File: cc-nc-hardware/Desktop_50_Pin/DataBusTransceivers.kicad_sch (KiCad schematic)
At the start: 38 parts, among them J1 Conn_01x03_Male, Q1 AO3401A, Q2 AO3401A, U3 AMS1117-2.85, U4 LVT245, U5 LVT245, U6 LVT245, U9 LVT245

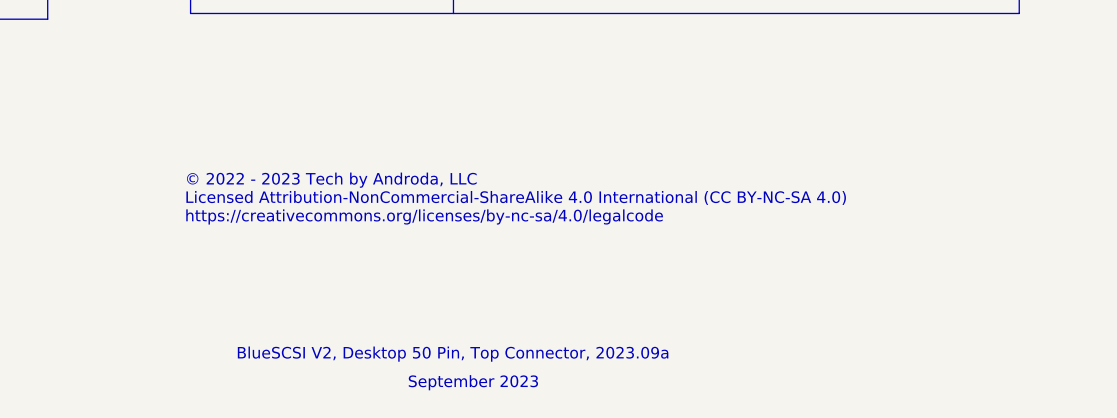
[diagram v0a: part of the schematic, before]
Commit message: Desktop 2023.10a design
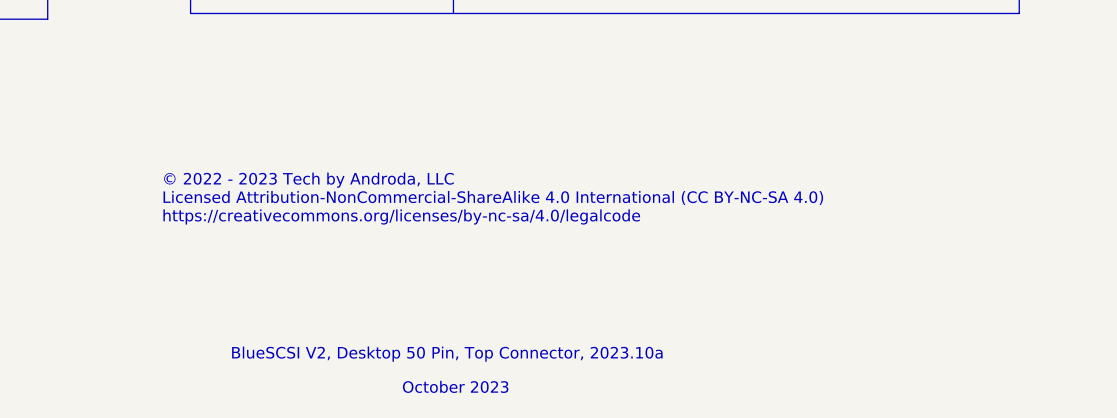
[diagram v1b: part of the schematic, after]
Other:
- note added: "BlueSCSI V2, Desktop 50 Pin, Top Connector, 2023.10a"
- note added: "October 2023"
- note removed: "BlueSCSI V2, Desktop 50 Pin, Top Connector, 2023.09a"
- note removed: "September 2023"
